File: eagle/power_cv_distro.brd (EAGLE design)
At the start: 101.6 x 80 mm, 54 parts, among them U1 POWER, U10 TLV2372IP, U11 TLV2372IP, U12 TLV2372IP, U13 TLV2372IP, U2 POWER, U3 POWER, U4 POWER, U5 POWER, U6 POWER, U7 POWER, U8 POWER, U9 POWER

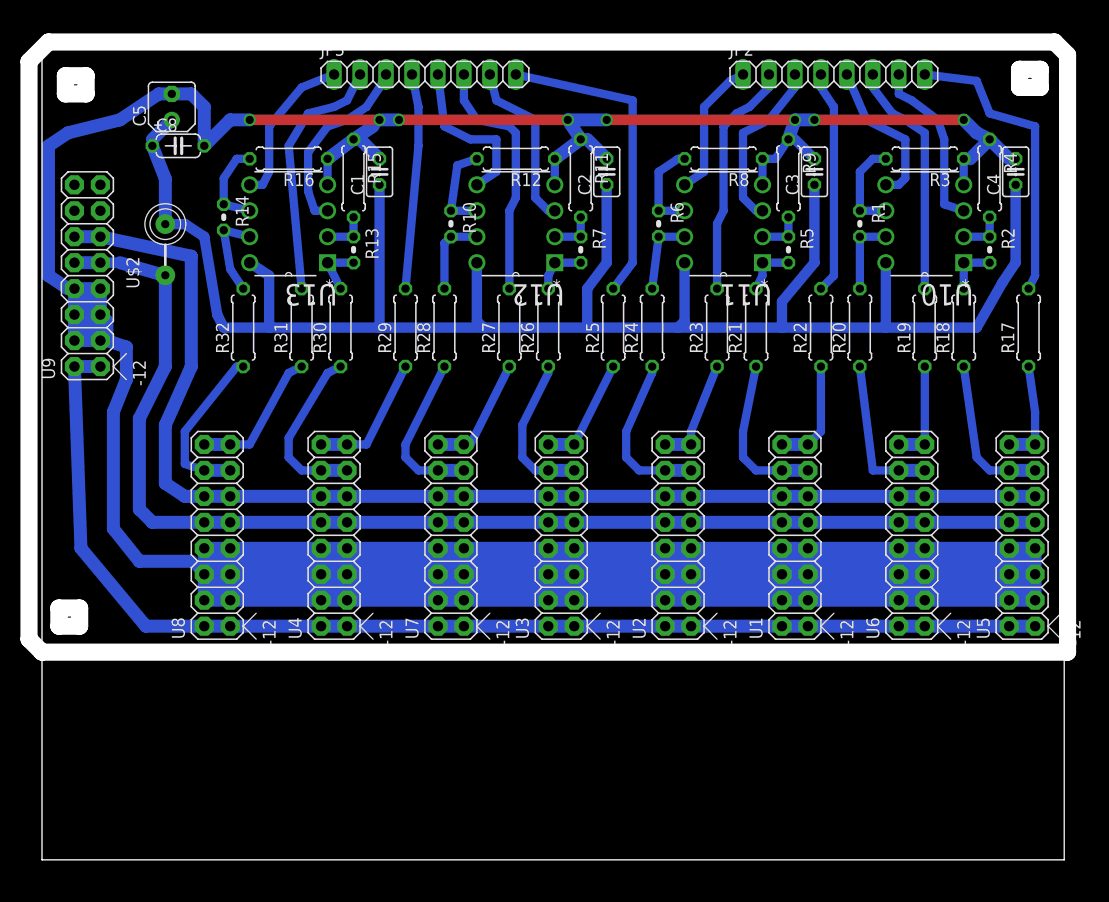
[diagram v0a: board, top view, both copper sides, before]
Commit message: power dist do-over begins
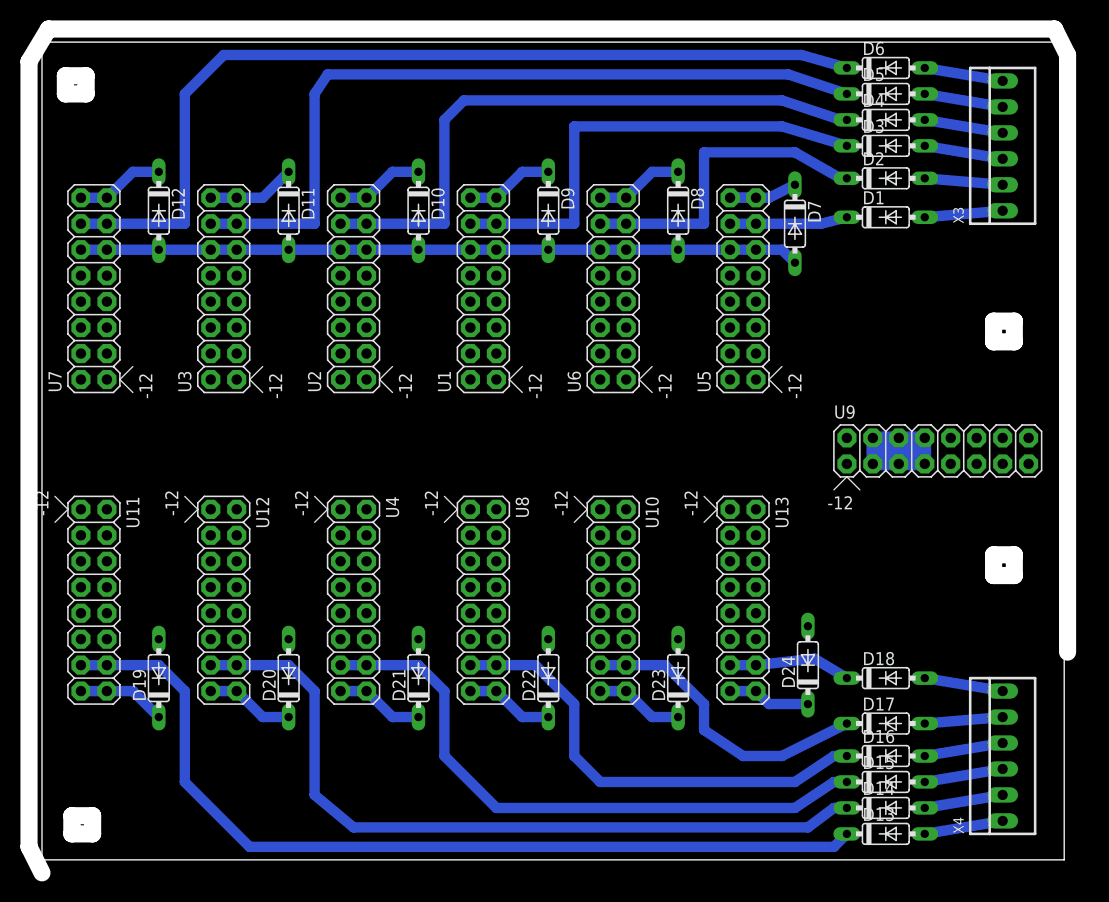
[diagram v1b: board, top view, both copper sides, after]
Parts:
- removed C1, C2, C3, C4: 100n, rcl:C025-025X050
- removed C5: 10u, rcl:B45181A
- removed C8: 100n, rcl:C050-024X044
- removed JP2, JP3: (no value), pinhead:1X08
- removed R1, R10, R13, R14, R2, R5, R6, R7: 1k8, rcl:0204V
- removed R11, R12, R15, R16, R17, R18, R19, R20, R21, R22, R23, R24, R25, R26, R27, R28, R29, R3, R30, R31, R32, R4, R8, R9: 1k, rcl:0207/7
- removed U$2: FB, adafruit:FB
- added D1, D10, D11, D12, D13, D14, D15, D16, D17, D18, D19, D2, D20, D21, D22, D23, D24, D3, D4, D5, D6, D7, D8, D9: 1N4148DO35-7, TR808clone:DO35-7
- added X3, X4: (no value), con-molex:22-23-2061
- U10, U11, U12, U13: value TLV2372IP -> POWER; device Texas Instruments_By_element14_Batch_1:DIP254P762X508-8 -> eurorack:POWER_16
- moved U9 82.0 mm to (85.1, 40.0), turned to 0 degrees
- moved U11 69.2 mm to (5.08, 27.9), turned to 270 degrees
- moved U13 61.5 mm to (68.6, 27.9), turned to 270 degrees
- moved U10 46.5 mm to (55.9, 27.9), turned to 270 degrees
- moved U12 45.4 mm to (17.8, 27.9), turned to 270 degrees
- moved U7 42.5 mm to (5.08, 53.3)
- moved U3 40.9 mm to (17.8, 53.3)
- moved U2 39.9 mm to (30.5, 53.3)
- moved U1 38.9 mm to (43.2, 53.3)
- moved U6 37.9 mm to (55.9, 53.3)
- moved U5 36.4 mm to (68.6, 53.3)
- moved U8 26.1 mm to (43.2, 27.9), turned to 270 degrees
- moved U4 2.29 mm to (30.5, 27.9), turned to 270 degrees
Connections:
- removed net N$37: R22.1, U1.15, U1.16
- removed net N$38: R21.1, U1.13, U1.14
- removed net N$39: R23.1, U2.15, U2.16
- removed net N$40: R24.1, U2.13, U2.14
- removed net N$41: R25.1, U3.15, U3.16
- removed net N$42: R26.1, U3.13, U3.14
- removed net N$43: R27.1, U7.15, U7.16
- removed net N$44: R28.1, U7.13, U7.14
- removed net N$45: R29.1, U4.15, U4.16
- removed net N$46: R30.1, U4.13, U4.14
- removed net N$47: R31.1, U8.15, U8.16
- removed net N$48: R32.1, U8.13, U8.14
- removed net VDD: C1.1, C2.1, C3.1, C4.1, C5.+, C8.1, U$2.P$2, U10.8, U11.8, U12.8, U13.8
- net +12V: no longer U$2.P$1
- net +5V: now also D10.A, D11.A, D12.A, D19.A, D20.A, D21.A, D22.A, D23.A, D24.A, D7.A, D8.A, D9.A, U10.11, U10.12, U11.11, U11.12, U12.11, U12.12, U13.11, U13.12
- net -12V: now also U10.1, U10.2, U11.1, U11.2, U12.1, U12.2, U13.1, U13.2
- net GND: now also U10.3, U10.5, U10.6, U10.7, U10.8, U11.3, U11.5, U11.6, U11.7, U11.8, U12.3, U12.5, U12.6, U12.7, U12.8, U13.3, U13.5, U13.6, U13.7, U13.8; no longer C1.2, C2.2, C3.2, C4.2, C5.-, C8.2, R11.1, R12.1, R15.1, R16.1, R3.1, R4.1, R8.1, R9.1
- net N$1: now also D1.A, X3.1; no longer JP2.8, R17.2
- net N$10: now also D4.C, U2.13, U2.14; no longer JP3.7, U12.3
- net N$11: now also D5.C, U3.13, U3.14; no longer JP3.6, R27.2
- net N$12: now also D6.C, U7.13, U7.14; no longer JP3.5, U12.5
- net N$13: now also D7.C, U5.15, U5.16; no longer JP3.4, R29.2
- net N$14: now also D8.C, U6.15, U6.16; no longer R10.2, R28.2, U12.7
- net N$15: now also D9.C, U1.15, U1.16; no longer JP3.2, R31.2
- net N$16: now also D10.C, U2.15, U2.16; no longer JP3.1, U13.5
- net N$17: now also D11.C, U3.15, U3.16; no longer R1.2, R20.2, U10.7
- net N$18: now also D12.C, U7.15, U7.16; no longer R18.2, R2.2, U10.1
- net N$19: now also D13.A, X4.1; no longer R1.1, R3.2, U10.6
- net N$2: now also D2.A, X3.2; no longer JP2.7, U10.3
- net N$20: now also D14.A, X4.2; no longer R2.1, R4.2, U10.2
- net N$21: now also D15.A, X4.3; no longer R11.2, R7.1, U12.2
- net N$22: now also D17.A, X4.5; no longer R24.2, R6.2, U11.7
- net N$23: now also D18.A, X4.6; no longer R5.1, R9.2, U11.2
- net N$24: now also D16.A, X4.4; no longer R6.1, R8.2, U11.6
- net N$25: now also D13.C, U11.13, U11.14; no longer R10.1, R12.2, U12.6
- net N$26: now also D14.C, U12.13, U12.14; no longer R21.2, R5.2, U11.1
- net N$27: now also D15.C, U4.13, U4.14; no longer R26.2, R7.2, U12.1
- net N$28: now also D16.C, U8.13, U8.14; no longer R13.2, R30.2, U13.1
- net N$29: now also D17.C, U10.13, U10.14; no longer R14.2, R32.2, U13.7
- net N$3: now also D3.A, X3.3; no longer JP2.6, R19.2
- net N$30: now also D18.C, U13.13, U13.14; no longer JP3.3, U13.3
- net N$31: now also D19.C, U11.15, U11.16; no longer R13.1, R15.2, U13.2
- net N$32: now also D20.C, U12.15, U12.16; no longer R14.1, R16.2, U13.6
- net N$33: now also D21.C, U4.15, U4.16; no longer R17.1, U5.15, U5.16
- net N$34: now also D22.C, U8.15, U8.16; no longer R18.1, U5.13, U5.14
- net N$35: now also D23.C, U10.15, U10.16; no longer R20.1, U6.13, U6.14
- net N$36: now also D24.C, U13.15, U13.16; no longer R19.1, U6.15, U6.16
- net N$4: now also D4.A, X3.4; no longer JP2.5, U10.5
- net N$49: now also U10.10, U10.9, U11.10, U11.9, U12.10, U12.9, U13.10, U13.9
- net N$5: now also D5.A, X3.5; no longer JP2.4, R22.2
- net N$6: now also D6.A, X3.6; no longer JP2.3, U11.3
- net N$7: now also D1.C, U5.13, U5.14; no longer JP2.2, R23.2
- net N$8: now also D2.C, U6.13, U6.14; no longer JP2.1, U11.5
- net N$9: now also D3.C, U1.13, U1.14; no longer JP3.8, R25.2
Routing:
- net GND: track 203.8 -> 0.00 mm, vias 8 -> 0
- net VDD: track 183.9 -> 0.00 mm
- net -12V: track 117.2 -> 0.00 mm
- net N$49: track 116.2 -> 0.00 mm
- net N$25: track 9.04 -> 88.0 mm
- net N$12: track 16.0 -> 89.4 mm
- net N$26: track 5.23 -> 75.2 mm
- net N$27: track 5.23 -> 59.8 mm
- net N$11: track 24.4 -> 76.3 mm
- net +5V: track 119.9 -> 70.4 mm
- net N$10: track 16.9 -> 60.8 mm
- net N$28: track 5.38 -> 45.3 mm
- net N$1: track 29.2 -> 7.65 mm
- net N$29: track 8.77 -> 29.8 mm
- net N$8: track 13.7 -> 31.8 mm
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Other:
- board size 101.6 x 80 mm -> 101.6 x 82.5 mm
